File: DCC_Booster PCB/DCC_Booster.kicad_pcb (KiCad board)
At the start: 2 copper layers, 96 parts, among them J1 Conn_01x04, J2 4P4C, J3 4P4C, J4 Prog, J5 Jack-DC, Q1 Q_NMOS_GDS, Q2 Q_NMOS_GDS, Q3 Q_NMOS_GDS, Q4 Q_NMOS_GDS, SW1 SW_DIP_x05, U1 MC34167, U10 LM358, U11 74AHC1G04, U2 R-78E5.0-1.0, U3 74HC08, U4 IR2101, U5 IR2101, U6 74AHC1G04, U7 6N137, U8 PIC16F1847-IP, U9 74AHC1G86

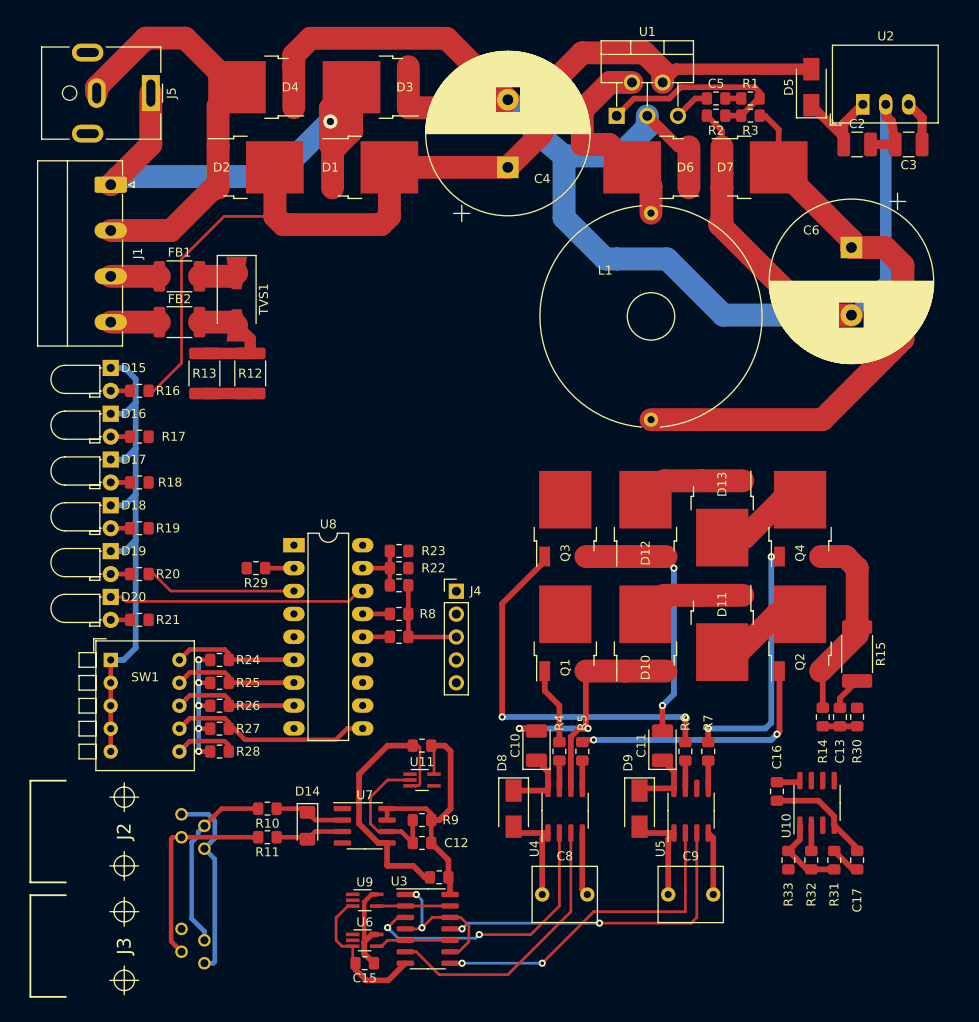
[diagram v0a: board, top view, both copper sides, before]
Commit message: pcb almost done
needs labels
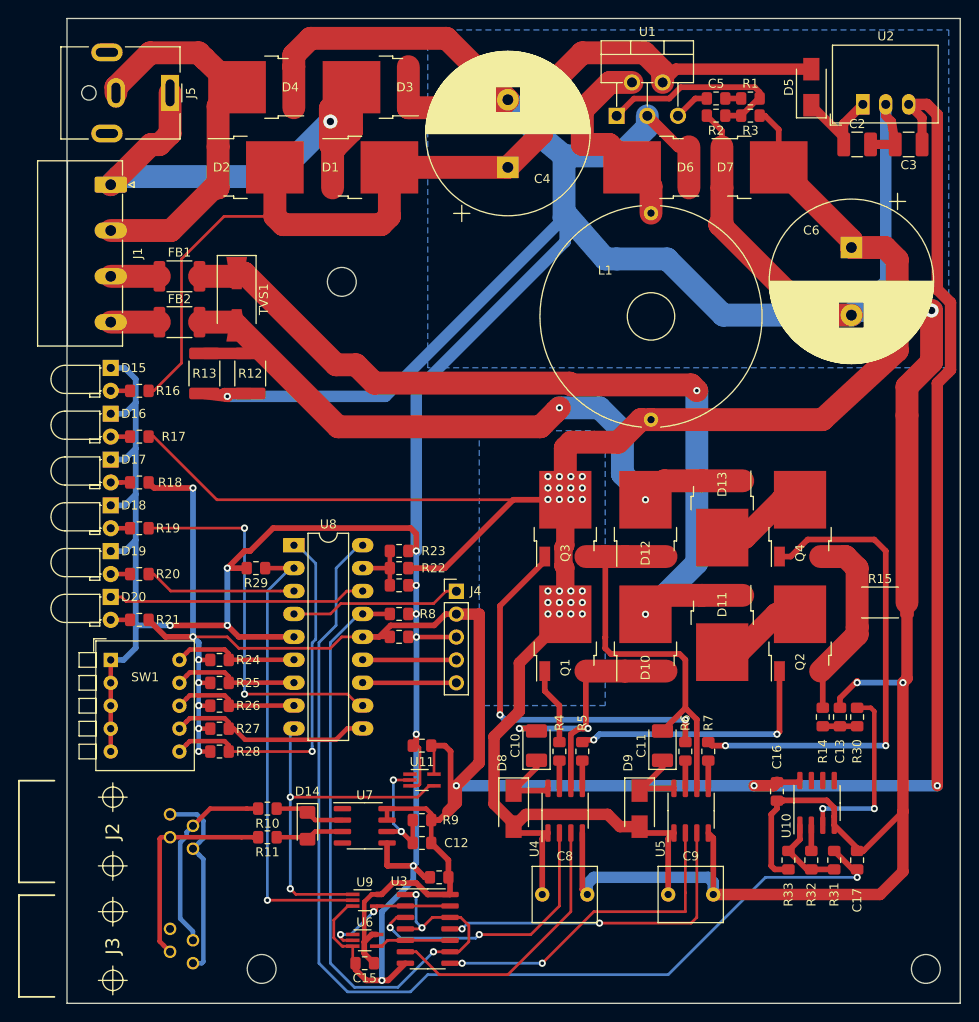
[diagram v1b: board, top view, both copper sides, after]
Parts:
- added H1: MountingHole_3.2mm_M3, MountingHole:MountingHole_3.2mm_M3, F.Cu at (130.8, 133.3)
- added H2: MountingHole_3.2mm_M3, MountingHole:MountingHole_3.2mm_M3, F.Cu at (57.1, 133.3)
- added H3: MountingHole_3.2mm_M3, MountingHole:MountingHole_3.2mm_M3, F.Cu at (66.0, 57.1)
- moved R15 6.25 mm to (125.7, 92.7), turned to 0 degrees
- moved J5 2.14 mm to (47.0, 36.2)
- moved J2 1.27 mm to (40.6, 118.1)
- moved J3 1.27 mm to (40.6, 130.8)
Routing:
- net GND: track 340.5 -> 648.6 mm, vias 0 -> 14
- net +5V: track 69.0 -> 300.8 mm, vias 5 -> 10
- net +15V: track 87.9 -> 223.7 mm, vias 0 -> 24
- net Net-(C17-Pad1): track 3.39 -> 119.1 mm, vias 0 -> 1
- net Net-(D10-Pad2): track 15.9 -> 99.5 mm, vias 0 -> 2
- net Net-(D12-Pad2): track 24.7 -> 82.8 mm, vias 0 -> 2
- net DCC_Enable: track 20.5 -> 76.9 mm, vias 2 -> 3
- net DCC_POL: track 3.19 -> 50.9 mm, vias 0 -> 1
- net Drv_Status: track 0.00 -> 42.7 mm, vias 0 -> 2
- net DCC_Sig: track 0.00 -> 41.6 mm, vias 0 -> 2
- net TestMode: track 6.84 -> 40.4 mm, vias 0 -> 1
- net Net-(Q4-Pad1): track 28.1 -> 54.5 mm
- net Net-(R30-Pad2): track 0.00 -> 20.4 mm, vias 0 -> 2
- net VPP: track 0.00 -> 19.1 mm
- net Net-(C11-Pad2): track 29.1 -> 46.9 mm, vias 2 -> 0
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- added copper zone on B.Cu, net +15V
- added copper zone on B.Cu, net GND
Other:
- board outline added: 99.1 x 109.2 mm
